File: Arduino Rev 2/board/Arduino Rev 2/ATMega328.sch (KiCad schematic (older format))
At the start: 1 part, among them U201 ATMEGA328-AU

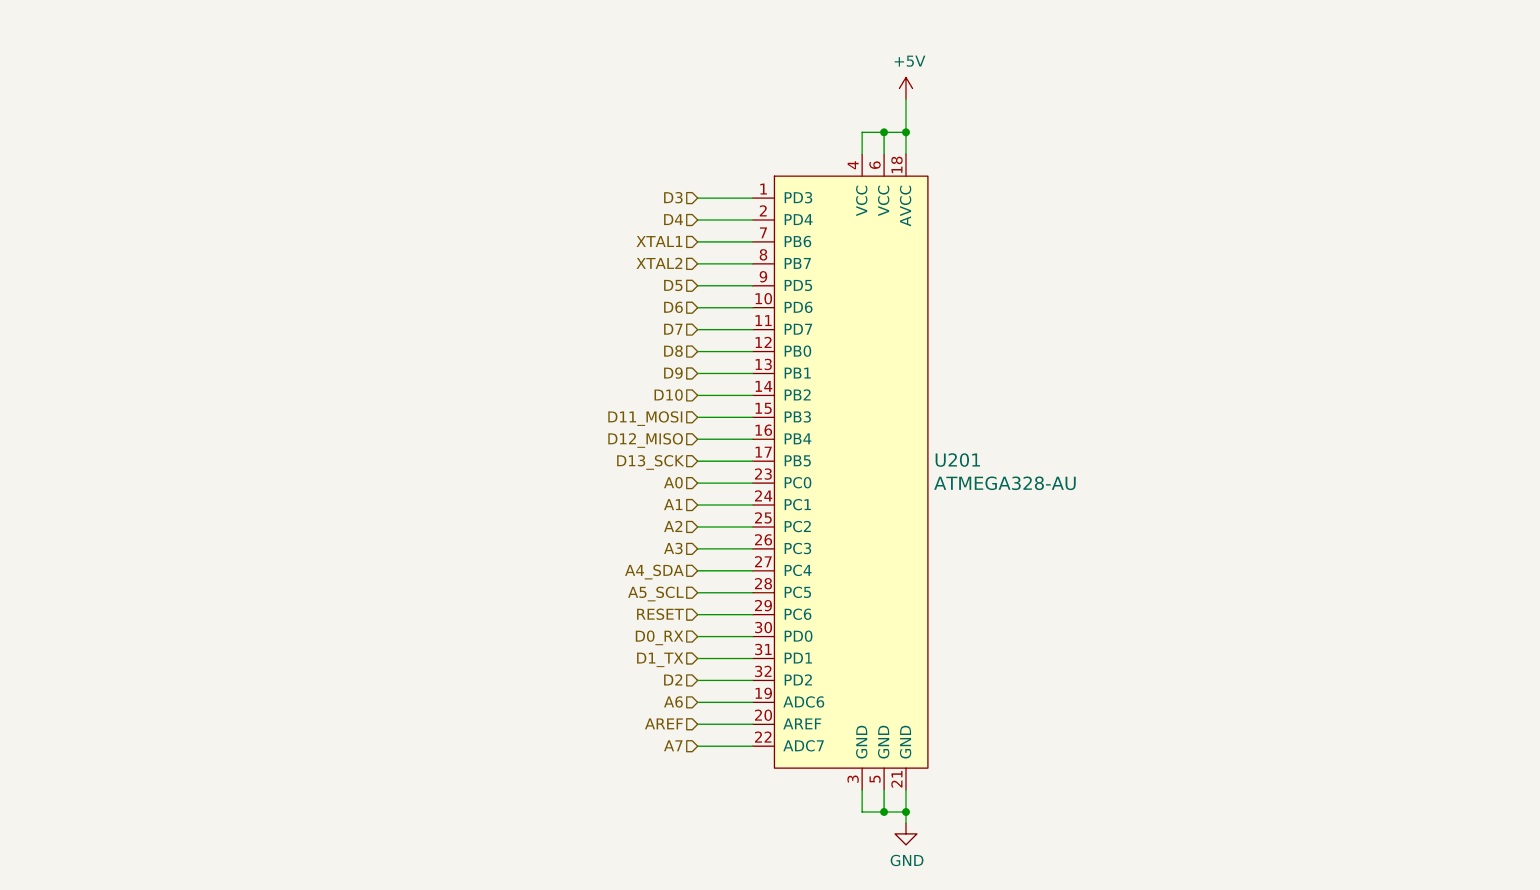
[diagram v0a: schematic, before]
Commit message: finished Schematic
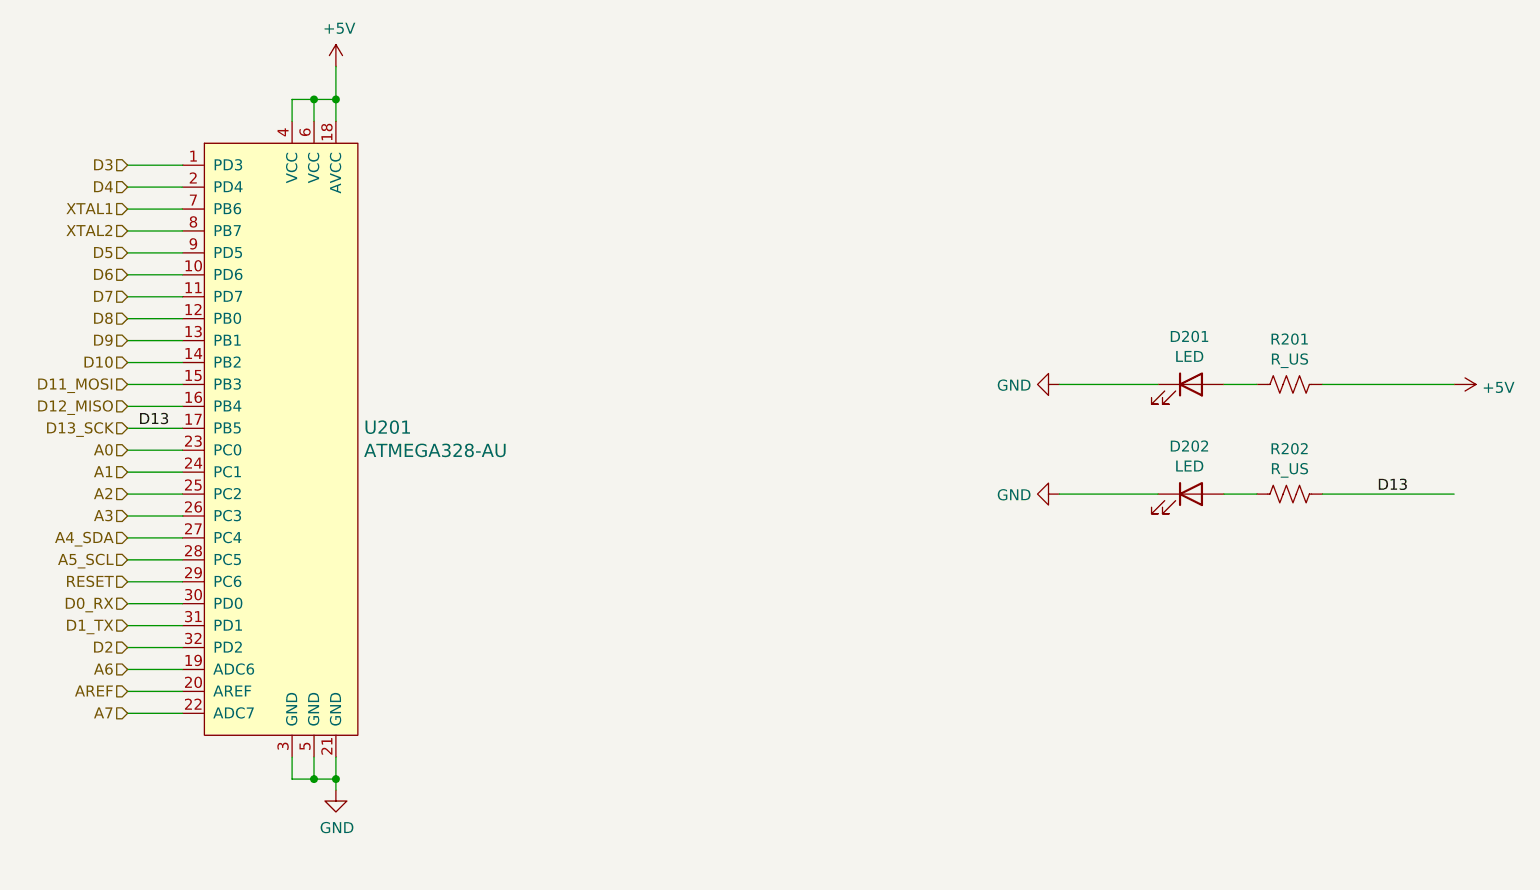
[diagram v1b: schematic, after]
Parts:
- added D201, D202: LED, Arduino Rev 2:led, symbol arduino_symbols:LED
- added R201, R202: R_US, Arduino Rev 2:R_0603_1608Metric_Pad1.05x0.95mm_HandSolder, symbol arduino_symbols:R_US
- U201: footprint digikey-footprints:TQFP-32_7x7mm -> Arduino Rev 2:TQFP-32_7x7mm
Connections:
- net +5V: now also R201.1
- net D13_SCK: now also R202.1
- net GND: now also D201.1 (K), D202.1 (K)
- new net: D201.2 (A), R201.2
- new net: D202.2 (A), R202.2
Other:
- moved on the sheet: U201
